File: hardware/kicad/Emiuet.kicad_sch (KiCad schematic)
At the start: 261 parts, among them J1 USB_C_Receptacle_USB2.0_16P, J2 USB_C_Receptacle_USB2.0_16P, J3 AudioJack3, J4 Conn_01x02_Pin, Q1 S9013 J3, SW1 SW_Slide_DPDT, SW1_0 Switch_SW_Push, SW1_1 Switch_SW_Push, SW1_10 Switch_SW_Push, SW1_11 Switch_SW_Push, SW1_12 Switch_SW_Push, SW1_2 Switch_SW_Push, SW1_3 Switch_SW_Push, SW1_4 Switch_SW_Push, SW1_5 Switch_SW_Push, SW1_6 Switch_SW_Push, SW1_7 Switch_SW_Push, SW1_8 Switch_SW_Push, SW1_9 Switch_SW_Push, SW2 SW_SPST, SW2_0 Switch_SW_Push, SW2_1 Switch_SW_Push, SW2_10 Switch_SW_Push, SW2_11 Switch_SW_Push, SW2_12 Switch_SW_Push, SW2_2 Switch_SW_Push, SW2_3 Switch_SW_Push, SW2_4 Switch_SW_Push, SW2_5 Switch_SW_Push, SW2_6 Switch_SW_Push, SW2_7 Switch_SW_Push, SW2_8 Switch_SW_Push, SW2_9 Switch_SW_Push, SW3 SW_SPST, SW3_0 Switch_SW_Push, SW3_1 Switch_SW_Push, SW3_10 Switch_SW_Push, SW3_11 Switch_SW_Push, SW3_12 Switch_SW_Push, SW3_2 Switch_SW_Push, SW3_3 Switch_SW_Push, SW3_4 Switch_SW_Push, SW3_5 Switch_SW_Push, SW3_6 Switch_SW_Push, SW3_7 Switch_SW_Push, SW3_8 Switch_SW_Push, SW3_9 Switch_SW_Push, SW4 SW_SPST, SW4_0 Switch_SW_Push, SW4_1 Switch_SW_Push, SW4_10 Switch_SW_Push, SW4_11 Switch_SW_Push, SW4_12 Switch_SW_Push, SW4_2 Switch_SW_Push, SW4_3 Switch_SW_Push, SW4_4 Switch_SW_Push, SW4_5 Switch_SW_Push, SW4_6 Switch_SW_Push, SW4_7 Switch_SW_Push, SW4_8 Switch_SW_Push, SW4_9 Switch_SW_Push, SW5_0 Switch_SW_Push, SW5_1 Switch_SW_Push, SW5_10 Switch_SW_Push, SW5_11 Switch_SW_Push, SW5_12 Switch_SW_Push, SW5_2 Switch_SW_Push, SW5_3 Switch_SW_Push, SW5_4 Switch_SW_Push, SW5_5 Switch_SW_Push, SW5_6 Switch_SW_Push, SW5_7 Switch_SW_Push, SW5_8 Switch_SW_Push, SW5_9 Switch_SW_Push, SW6_0 Switch_SW_Push, SW6_1 Switch_SW_Push, SW6_10 Switch_SW_Push, SW6_11 Switch_SW_Push, SW6_12 Switch_SW_Push, SW6_2 Switch_SW_Push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

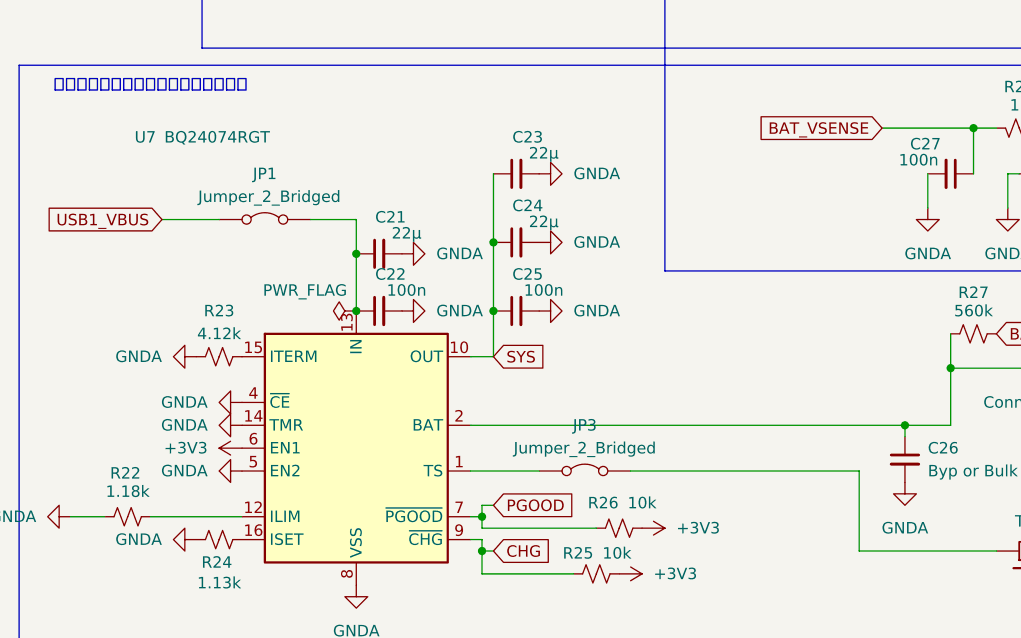
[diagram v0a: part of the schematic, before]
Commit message: Fix Kicad Data
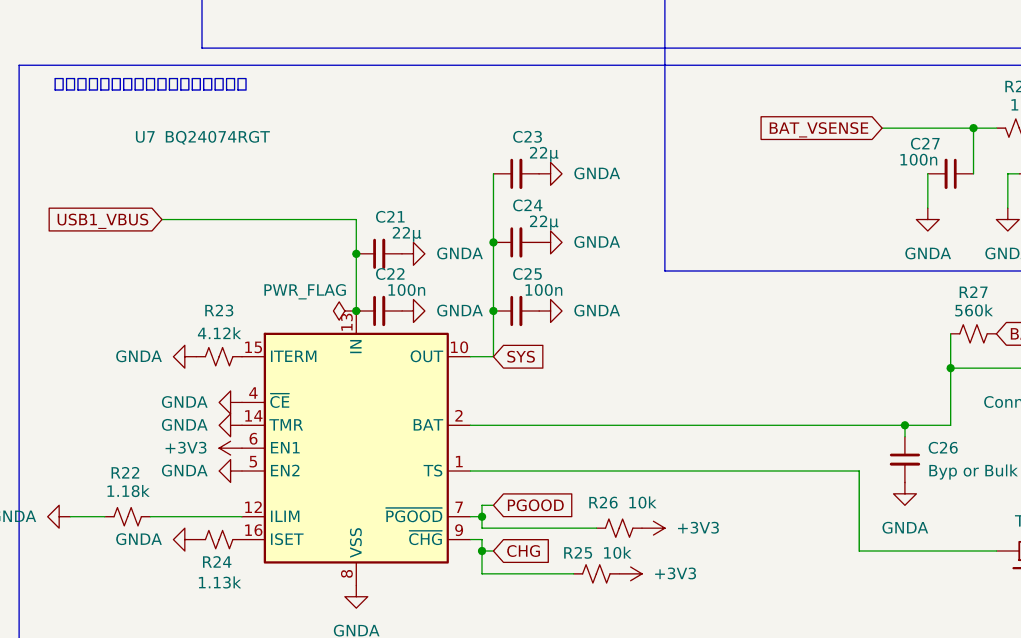
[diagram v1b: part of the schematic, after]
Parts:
- removed JP1: Jumper_2_Bridged, TestPoint:TestPoint_2Pads_Pitch2.54mm_Drill0.8mm, symbol Jumper:Jumper_2_Bridged
- removed JP3: Jumper_2_Bridged, Jumper:SolderJumper-2_P1.3mm_Bridged_RoundedPad1.0x1.5mm, symbol Jumper:Jumper_2_Bridged
- BT1: footprint EUB_Passives:Battery Cell 800mah bis -> EUB_Passives:Battery Cell 800mah nobis
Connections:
- net USB1_VBUS: now also C21.1, C22.1, U7.13 (IN)
- net at U7.1 (TS): now also TH1.1
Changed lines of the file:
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@@
 	(wire
 		(pts
-			(xy 271.78 204.47) (xy 278.13 204.47)
+			(xy 271.78 204.47) (xy 293.37 204.47)
 		)
 		(stroke
@@
 	(wire
 		(pts
-			(xy 306.07 232.41) (xy 313.69 232.41)
+			(xy 306.07 232.41) (xy 349.25 232.41)
 		)
 		(stroke
@@
 	(wire
 		(pts
-			(xy 288.29 204.47) (xy 293.37 204.47)
-		)
-		(stroke
-			(width 0)
-			(type default)
-		)
-	)
-	(wire
-		(pts
 			(xy 374.65 241.3) (xy 375.92 241.3)
 		)
@@
 	(wire
 		(pts
-			(xy 323.85 232.41) (xy 349.25 232.41)
-		)
-		(stroke
-			(width 0)
-			(type default)
-		)
-	)
-	(wire
-		(pts
 			(xy 318.77 66.04) (xy 318.77 69.85)
 		)
@@
 	)
 	(symbol
-		(lib_id "Jumper:Jumper_2_Bridged")
-		(at 318.77 232.41 0)
-		(unit 1)
-		(exclude_from_sim no)
-		(in_bom yes)
-		(on_board yes)
-		(dnp no)
-		(fields_autoplaced yes)
-		(property "Reference" "JP3"
-			(at 318.77 227.33 0)
-			(effects
-				(font
-					(size 1.27 1.27)
-				)
-			)
-		)
-		(property "Value" "Jumper_2_Bridged"
-			(at 318.77 229.87 0)
-			(effects
-				(font
-					(size 1.27 1.27)
-				)
-			)
-		)
-		(property "Footprint" "Jumper:SolderJumper-2_P1.3mm_Bridged_RoundedPad1.0x1.5mm"
-			(at 318.77 232.41 0)
-			(effects
-				(font
-					(size 1.27 1.27)
-				)
-				(hide yes)
-			)
-		)
-		(property "Datasheet" "~"
-			(at 318.77 232.41 0)
-			(effects
-				(font
-					(size 1.27 1.27)
-				)
-				(hide yes)
-			)
-		)
-		(property "Description" "Jumper, 2-pole, closed/bridged"
-			(at 318.77 232.41 0)
-			(effects
-				(font
-					(size 1.27 1.27)
-				)
-				(hide yes)
-			)
-		)
-		(pin "1"
-		)
-		(pin "2"
-		)
-		(instances
-			(project ""
-				(path "/c9191c2a-649b-4f9d-b8cd-0f4c3bb1b88c"
-					(reference "JP3")
-					(unit 1)
-				)
-			)
-		)
-	)
-	(symbol
 		(lib_name "D_Small_1")
 		(lib_id "Device:D_Small")
@@
 	)
 	(symbol
-		(lib_id "Jumper:Jumper_2_Bridged")
-		(at 283.21 204.47 0)
-		(unit 1)
-		(exclude_from_sim no)
-		(in_bom yes)
-		(on_board yes)
-		(dnp no)
-		(property "Reference" "JP1"
-			(at 283.21 199.39 0)
-			(effects
-				(font
-					(size 1.27 1.27)
-				)
-			)
-		)
-		(property "Value" "Jumper_2_Bridged"
-			(at 283.718 201.93 0)
-			(effects
-				(font
-					(size 1.27 1.27)
-				)
-			)
-		)
-		(property "Footprint" "TestPoint:TestPoint_2Pads_Pitch2.54mm_Drill0.8mm"
-			(at 283.21 204.47 0)
-			(effects
-				(font
-					(size 1.27 1.27)
-				)
-				(hide yes)
-			)
-		)
-		(property "Datasheet" "~"
-			(at 283.21 204.47 0)
-			(effects
-				(font
-					(size 1.27 1.27)
-				)
-				(hide yes)
-			)
-		)
-		(property "Description" "Jumper, 2-pole, closed/bridged"
-			(at 283.21 204.47 0)
-			(effects
-				(font
-					(size 1.27 1.27)
-				)
-				(hide yes)
-			)
-		)
-		(pin "2"
-		)
-		(pin "1"
-		)
-		(instances
-			(project ""
-				(path "/c9191c2a-649b-4f9d-b8cd-0f4c3bb1b88c"
-					(reference "JP1")
-					(unit 1)
-				)
-			)
-		)
-	)
-	(symbol
 		(lib_id "power:GNDA")
 		(at 345.44 149.86 0)
@@
 			)
 		)
-		(property "Footprint" "EUB_Passives:Battery Cell 800mah bis"
+		(property "Footprint" "EUB_Passives:Battery Cell 800mah nobis"
 			(at 386.08 223.52 0)
 			(effects
